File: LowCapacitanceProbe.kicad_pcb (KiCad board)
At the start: 2 copper layers, 25.1 x 19.4 mm, 40 parts, among them J2 SMA, J3 Barrel_Jack_Switch, Q1 BF998, U2 SPX3819M5-L-5-0

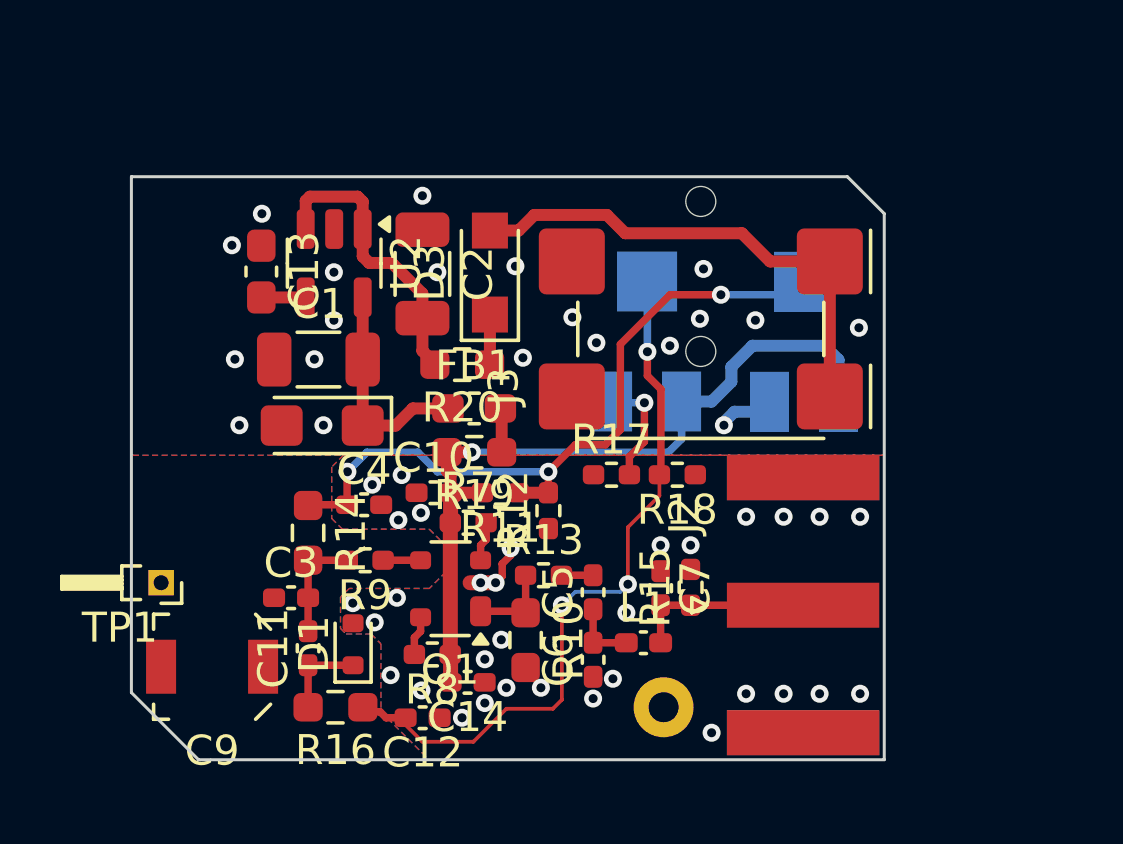
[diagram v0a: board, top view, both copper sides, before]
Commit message: More routing
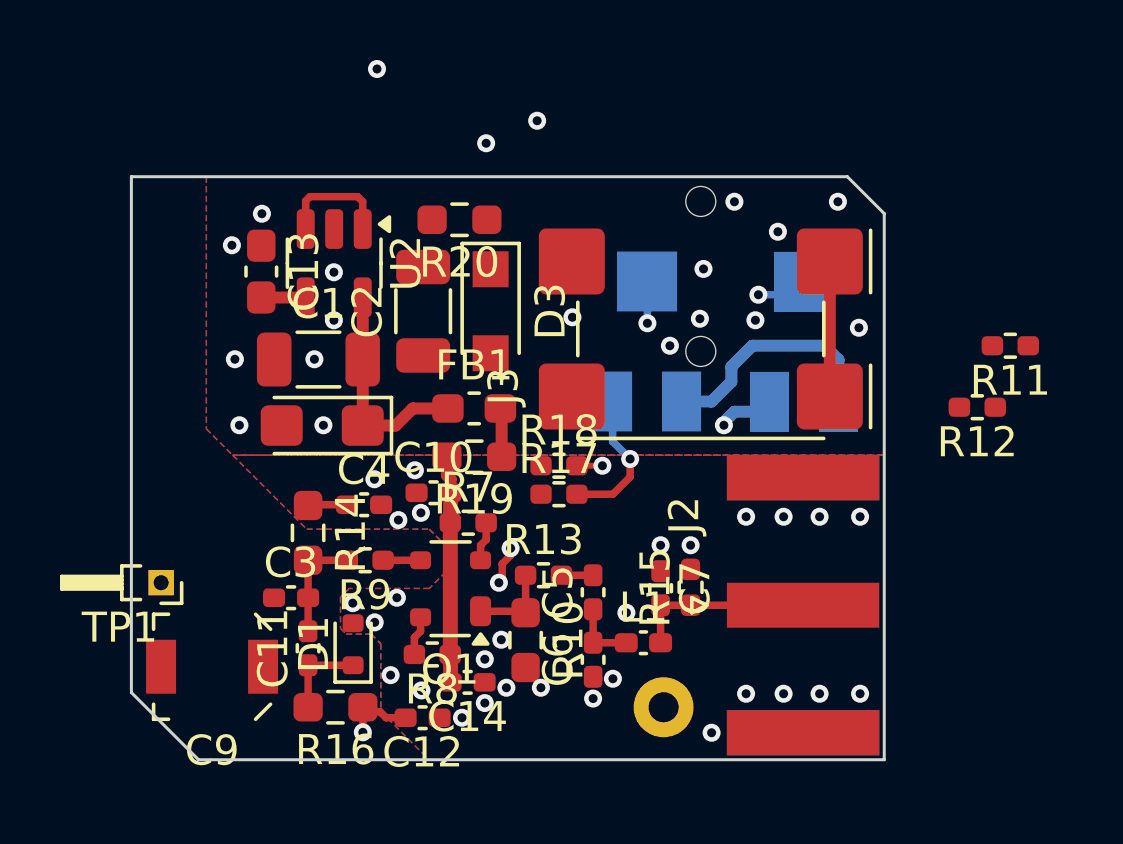
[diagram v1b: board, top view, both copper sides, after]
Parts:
- moved R11 17.7 mm to (141.9, 61.6)
- moved R12 14.7 mm to (140.8, 63.6), turned to 180 degrees
- moved R20 4.83 mm to (123.5, 57.4)
- moved R18 3.96 mm to (126.9, 65.6), turned to 0 degrees
- moved R17 1.87 mm to (126.9, 66.5)
- moved D3 1.29 mm to (124.6, 60.5), turned to -90 degrees
- moved C2 1.25 mm to (122.3, 60.5), turned to 90 degrees
- moved R19 0.15 mm to (124.0, 65.3)
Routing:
- net /G2_BIAS: track 24.2 -> 3.01 mm, vias 3 -> 1
- net /GAIN_TUNE: track 24.2 -> 10.1 mm
- net /PIN: track 16.7 -> 4.50 mm
- net /POWER: track 25.9 -> 15.5 mm, vias 1 -> 0
- net /PIN_FILT: track 9.83 -> 3.88 mm
- net Net-(D3-K): track 1.67 -> 0.00 mm
- net Net-(R17-Pad2): track 3.68 -> 4.77 mm
- net GND: track 14.3 -> 13.5 mm
- added copper zone on In1.Cu, net GND
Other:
- copper layers 2 -> 4
- rule pad_to_mask_clearance: 0.05 -> 0
